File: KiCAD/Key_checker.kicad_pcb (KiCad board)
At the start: 2 copper layers, 48.5 x 36 mm, 14 parts, among them Q1 Q_Photo_NPN, SW1 SW_DIP_x01, U1 ESP32-Dev-Module-ESP32-footpr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, U2 SSD1306

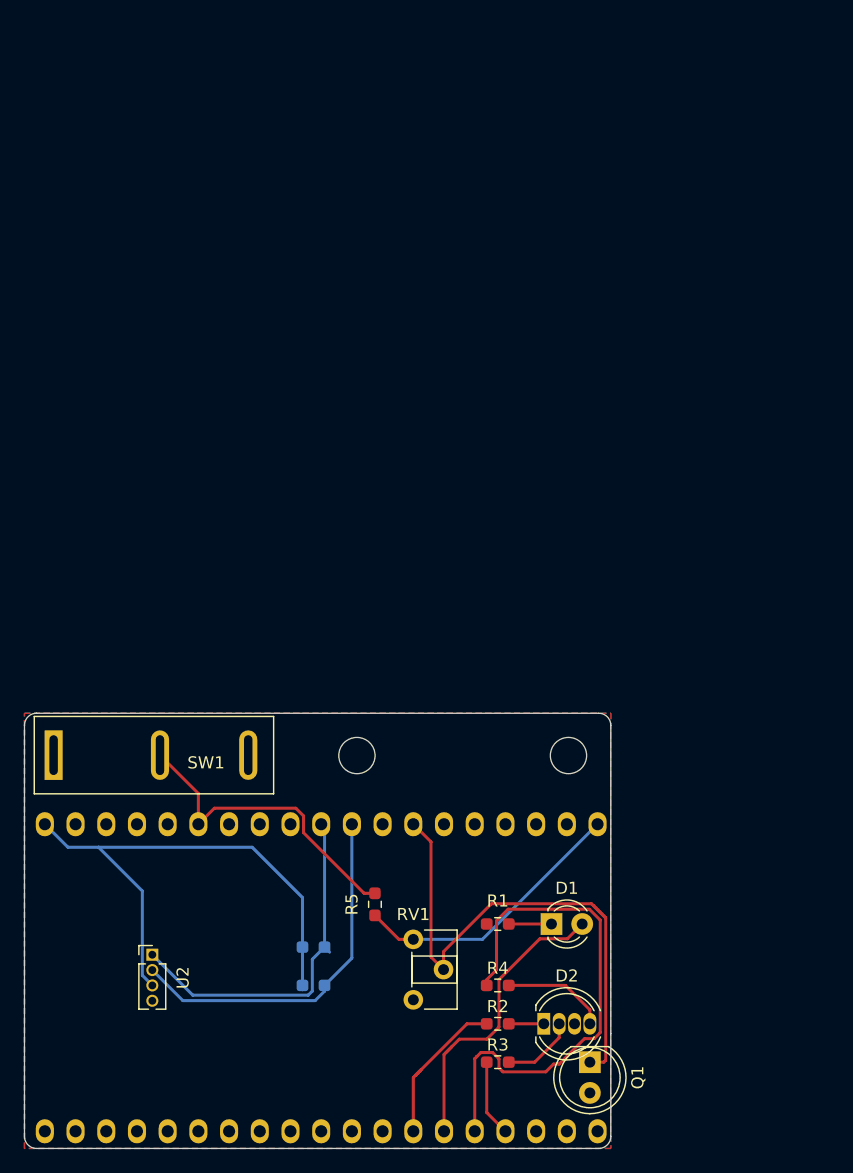
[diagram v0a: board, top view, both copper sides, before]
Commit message: Key Checker's PCB is Completed!
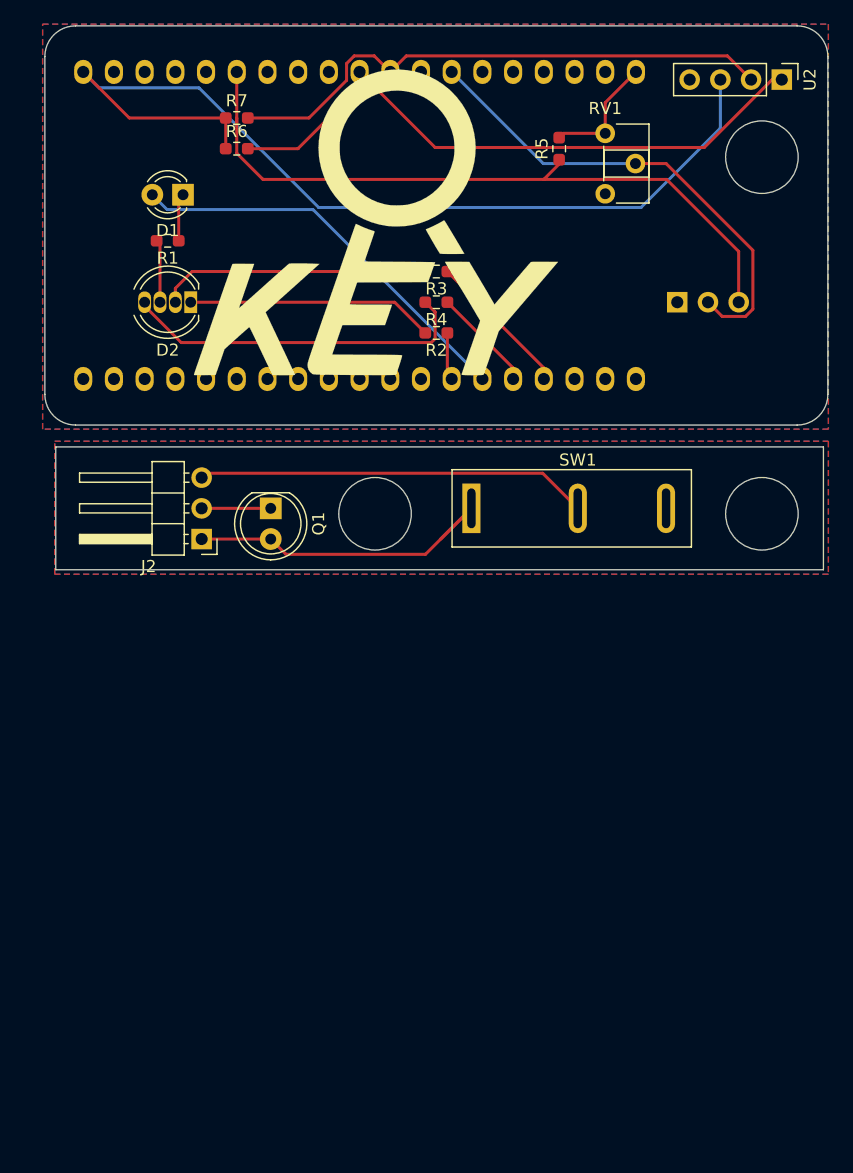
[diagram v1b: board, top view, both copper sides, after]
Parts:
- added G***: LOGO, other:Key_checker_logo, F.Cu at (174.0, 55.0)
- added J1: Conn_01x03_Male, Connector_PinHeader_2.54mm:PinHeader_1x03_P2.54mm_Horizontal, B.Cu at (199.0, 63.5)
- added J2: Conn_01x03_Male, Connector_PinHeader_2.54mm:PinHeader_1x03_P2.54mm_Horizontal, F.Cu at (159.7, 83.1)
- R6, R7: moved to F.Cu
- U1: value ESP32-Dev-Module-ESP32-footprints-Shem-Lib -> ESP32
- U2: footprint Connector_PinHeader_1.27mm:PinHeader_1x04_P1.27mm_Vertical -> Connector_PinHeader_2.54mm:PinHeader_1x04_P2.54mm_Vertical
- moved U2 89.2 mm to (207.6, 45.1), turned to 270 degrees
- moved R7 72.0 mm to (162.6, 48.3)
- moved RV1 68.5 mm to (193.0, 49.5)
- moved D1 67.6 mm to (158.1, 54.6), turned to 180 degrees
- moved D2 66.5 mm to (158.8, 63.5), turned to 180 degrees
- moved R6 66.3 mm to (162.6, 50.8)
- moved R3 65.6 mm to (179.1, 61.0), turned to 180 degrees
- moved R5 64.3 mm to (189.2, 50.8), turned to 90 degrees
- moved R1 62.8 mm to (156.8, 58.4)
- moved U1 62.3 mm to (172.7, 57.1)
- moved R2 57.4 mm to (179.1, 66.0), turned to 180 degrees
- moved R4 56.7 mm to (179.1, 63.5), turned to 180 degrees
- moved Q1 52.9 mm to (165.4, 80.5)
- moved SW1 40.1 mm to (190.8, 80.5)
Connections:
- net Net-(R5-Pad2) renamed +5V
- net Net-(R6-Pad1) renamed +3V3
- Q1 pad 1: Net-(Q1-Pad1) -> Net-(J2-Pad2)
- Q1 pad 2: GND -> Net-(J2-Pad1)
- R5 pad 1: Net-(R5-Pad1) -> Net-(J1-Pad3)
- RV1 pad 2: Net-(Q1-Pad1) -> Net-(J1-Pad2)
- SW1 pad 1: GND -> Net-(J2-Pad1)
- SW1 pad 2: Net-(R5-Pad1) -> Net-(J2-Pad3)
- U1 pad 13: Net-(Q1-Pad1) -> Net-(J1-Pad2)
- U1 pad 6: Net-(R5-Pad1) -> Net-(J1-Pad3)
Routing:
- net Net-(J1-Pad3): track 0.00 -> 58.3 mm
- net Net-(Q1-Pad1): track 44.7 -> 0.00 mm
- net Net-(J1-Pad2): track 0.00 -> 40.3 mm
- net +3V3: track 44.7 -> 80.0 mm
- net Net-(R4-Pad1): track 43.4 -> 8.60 mm
- net Net-(J2-Pad3): track 0.00 -> 32.5 mm
- net Net-(J2-Pad1): track 0.00 -> 28.0 mm
- net Net-(R5-Pad1): track 25.9 -> 0.00 mm
- net Net-(R6-Pad2): track 30.1 -> 52.4 mm
- net Net-(D2-Pad4): track 8.70 -> 29.1 mm
- net Net-(D2-Pad1): track 2.90 -> 20.5 mm
- net Net-(D2-Pad2): track 6.16 -> 22.4 mm
- net Net-(R7-Pad2): track 30.6 -> 46.5 mm
- net +5V: track 23.2 -> 10.1 mm
- net Net-(R2-Pad1): track 13.1 -> 3.96 mm
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- added copper zone on F.Cu, net (none)
- added copper zone on B.Cu, net Net-(J2-Pad1)
- added copper zone on F.Cu, net Net-(J2-Pad1)
- removed copper zone on F.Cu, net GND
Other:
- board size 48.5 x 36 mm -> 64.8 x 45 mm
